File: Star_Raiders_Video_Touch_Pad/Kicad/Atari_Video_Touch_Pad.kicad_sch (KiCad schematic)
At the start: 8 parts, among them J1 DE9, SW1 FORE_VIEW, SW2 GAL_MAP, SW3 HYPERWARP, SW4 COMPUTER_ON/OFF, SW5 SHIELDS_ON/OFF

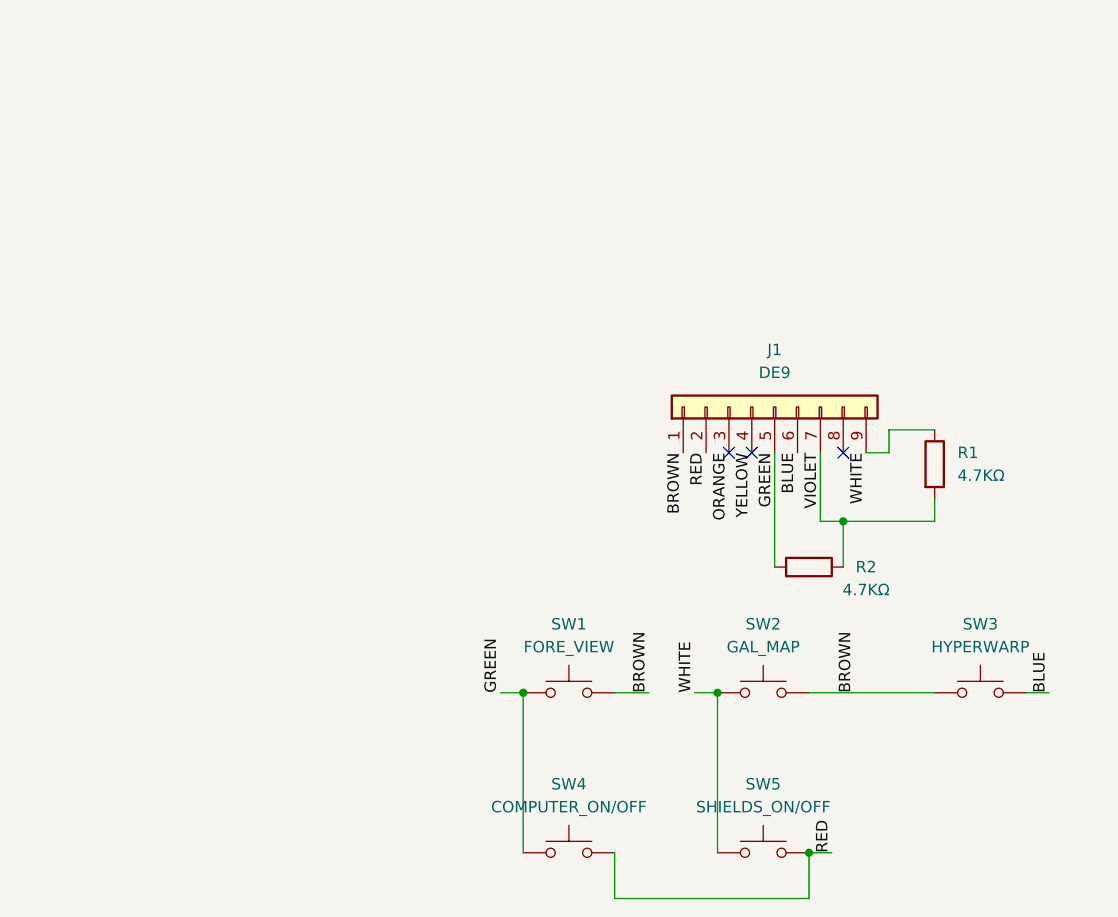
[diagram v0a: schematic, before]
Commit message: Improved design (maybe?)
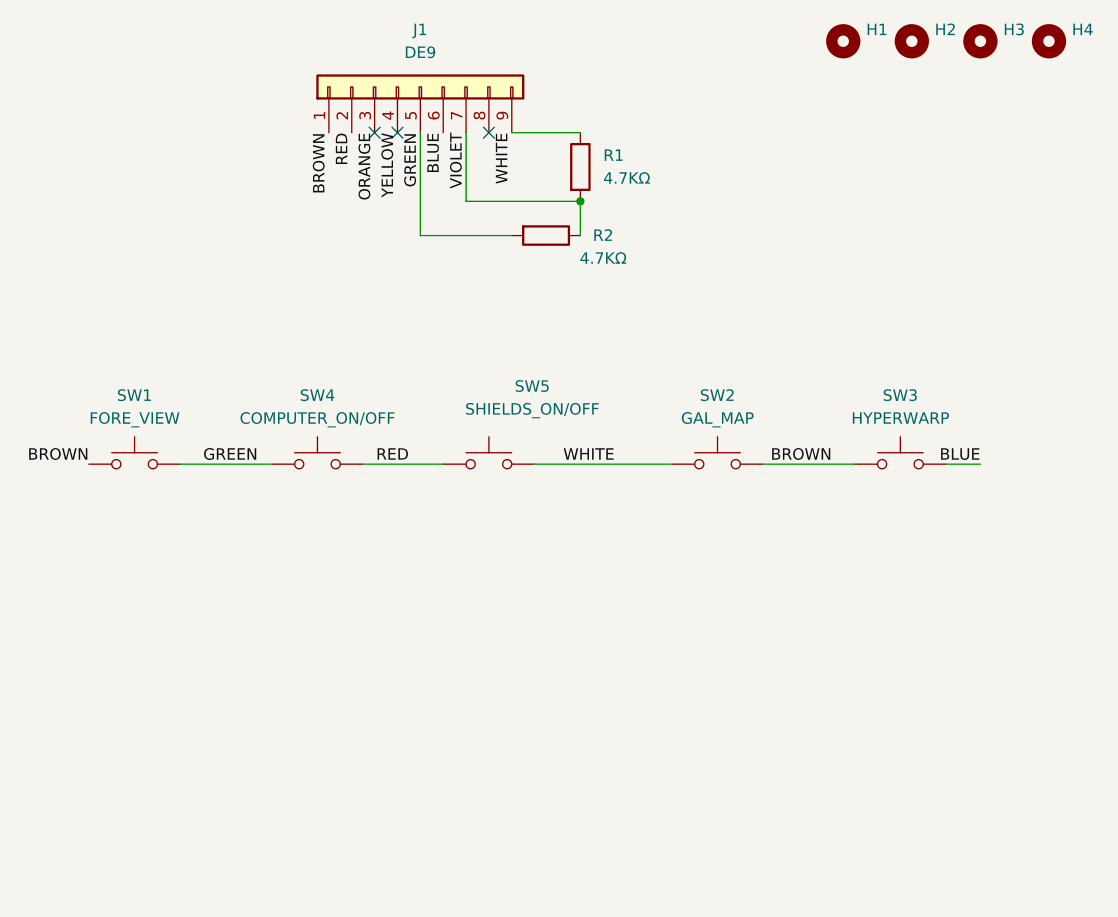
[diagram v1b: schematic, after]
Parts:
- added H1, H2, H3, H4: MountingHole, MountingHole:MountingHole_3.2mm_M3, symbol Mechanical:MountingHole
- SW1, SW2, SW3, SW4, SW5: footprint MX1A-11NW:MX1A11NW -> PCM_Switch_Keyboard_Cherry_MX:SW_Cherry_MX_PCB_1.00u
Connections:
- net BROWN: now also SW1.1; no longer SW1.2
- net GREEN: now also SW1.2; no longer SW1.1
- net RED: now also SW5.1; no longer SW5.2
- net WHITE: now also SW5.2; no longer SW5.1
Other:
- moved on the sheet: J1, R1, R2, SW1, SW2, SW3, SW4, SW5
